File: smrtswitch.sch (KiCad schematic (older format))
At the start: 8 parts, among them J1 Screw_Terminal_01x02, J2 Conn_01x08, J3 Conn_01x03, J4 Conn_01x03, J5 Conn_01x03, J6 Conn_01x03

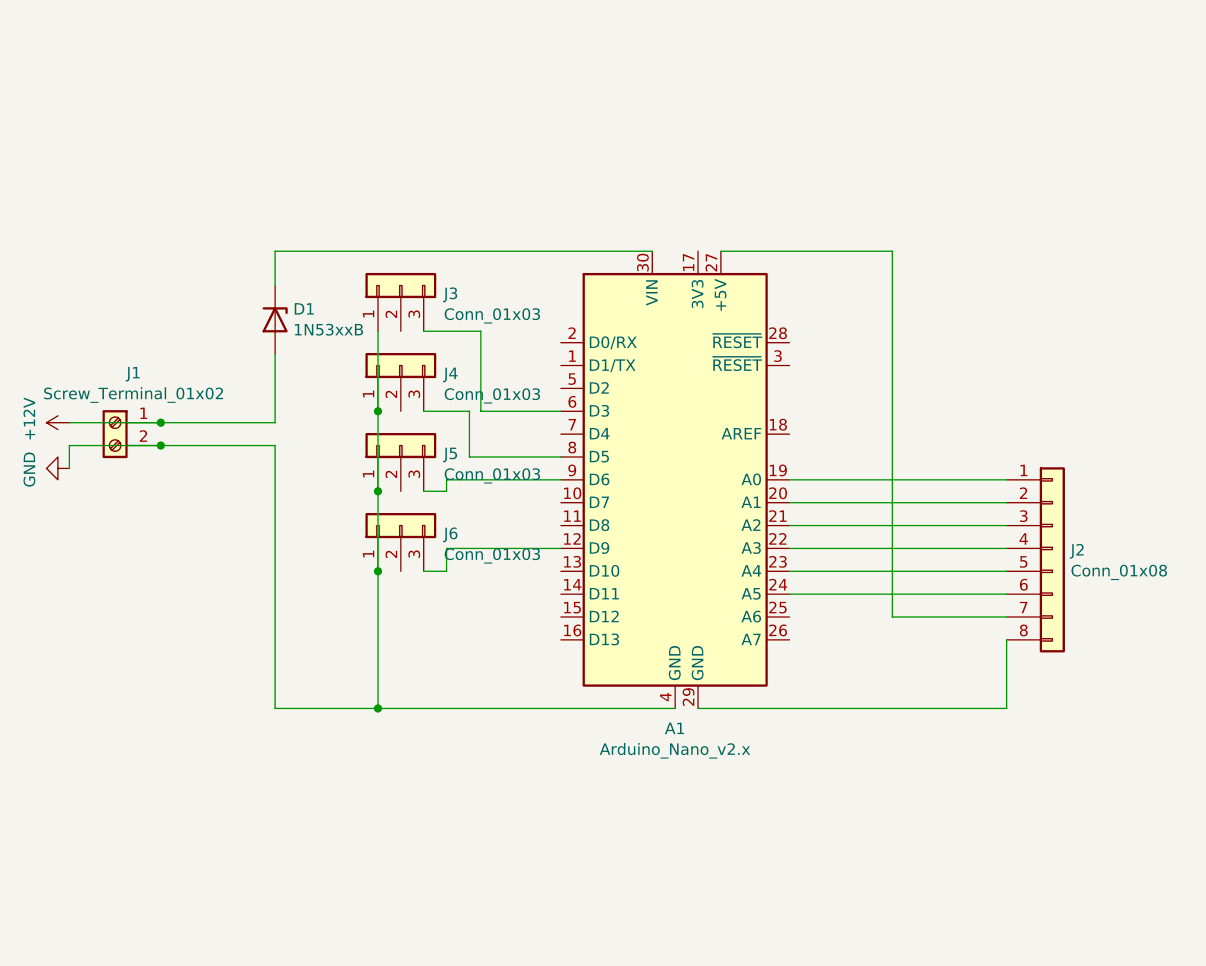
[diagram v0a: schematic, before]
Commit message: long-uncommitted changes
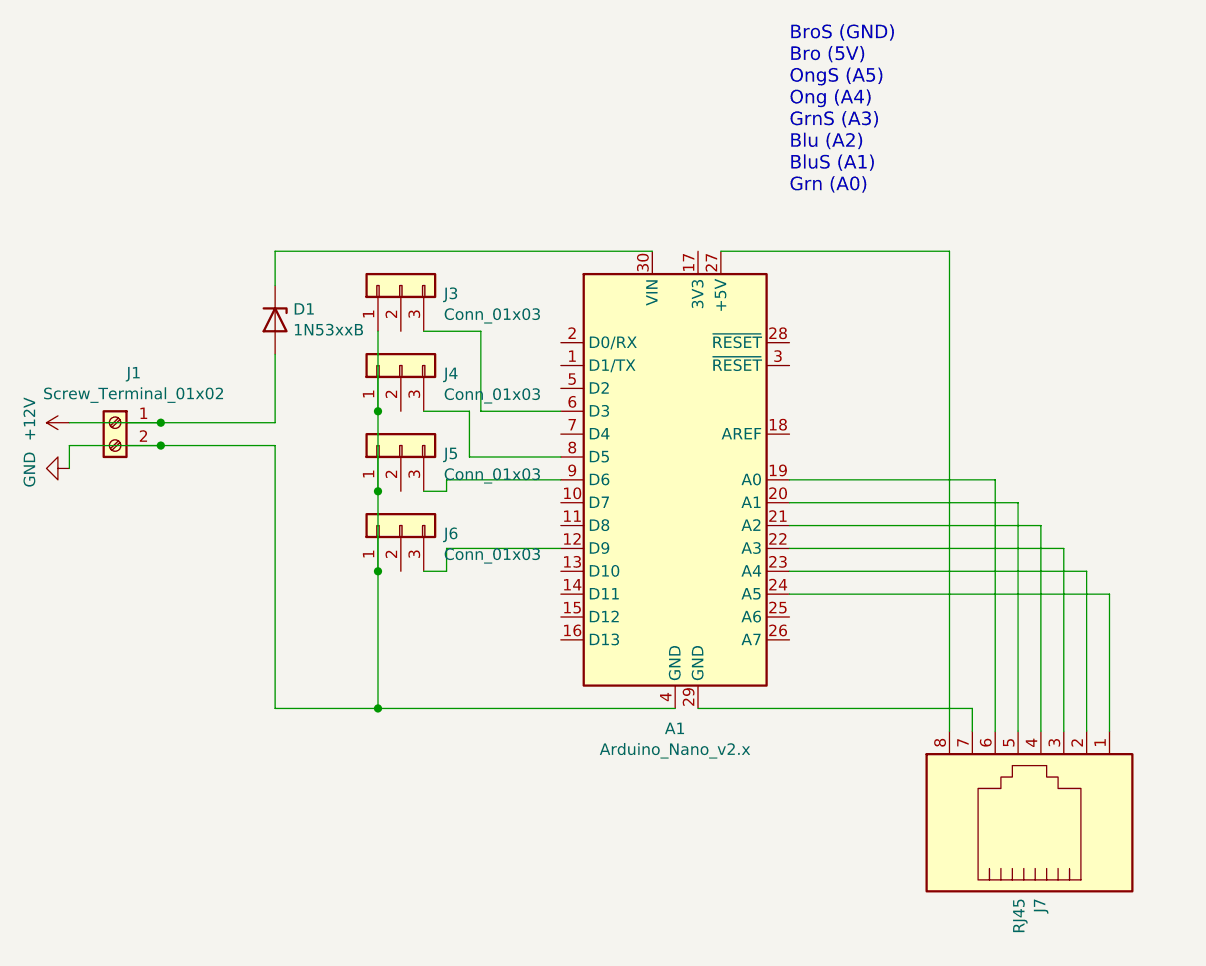
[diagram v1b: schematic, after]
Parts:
- removed J2: Conn_01x08, Connector_PinHeader_2.54mm:PinHeader_1x08_P2.54mm_Vertical, symbol Connector_Generic:Conn_01x08
- added J7: RJ45, Connector_RJ:RJ45_Amphenol_54602-x08_Horizontal, symbol Connector:RJ45
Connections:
- net at A1.19 (A0): now also J7.6
- net at A1.20 (A1): now also J7.5
- net at A1.21 (A2): now also J7.4
- net at A1.22 (A3): now also J7.3
- net at A1.23 (A4): now also J7.2
- net at A1.24 (A5): now also J7.1
- net at A1.27 (+5V): now also J7.8
- net at A1.29 (GND): now also J7.7
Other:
- note added: "BroS (GND)\nBro (5V)\nOngS (A5)\nOng (A4)\nGrnS (A3)\nBlu (A2)\nBluS (A1)\nGrn (A0)"
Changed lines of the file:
@@
 $EndComp
-$Comp
-L Connector_Generic:Conn_01x08 J2
-U 1 1 5E218367
-P 7100 3800
-F 0 "J2" H 7180 3792 50  0000 L CNN
-F 1 "Conn_01x08" H 7180 3701 50  0000 L CNN
-F 2 "Connector_PinHeader_2.54mm:PinHeader_1x08_P2.54mm_Vertical" H 7100 3800 50  0001 C CNN
-F 3 "~" H 7100 3800 50  0001 C CNN
-	1    7100 3800
-	1    0    0    -1
-$EndComp
-Wire Wire Line
-	5950 3500 6900 3500
-Wire Wire Line
-	6900 3600 5950 3600
-Wire Wire Line
-	5950 3700 6900 3700
-Wire Wire Line
-	6900 3800 5950 3800
-Wire Wire Line
-	5950 3900 6900 3900
-Wire Wire Line
-	6900 4000 5950 4000
-Wire Wire Line
-	5550 4500 6900 4500
-Wire Wire Line
-	6900 4500 6900 4200
-Wire Wire Line
-	5650 2500 6400 2500
-Wire Wire Line
-	6400 2500 6400 4100
-Wire Wire Line
-	6400 4100 6900 4100
 $Comp
 L Connector:Screw_Terminal_01x02 J1
@@
 Wire Wire Line
 	4150 3900 4150 4500
+$Comp
+L Connector:RJ45 J7
+U 1 1 5EEEE824
+P 7050 5000
+F 0 "J7" H 6720 5004 50  0000 R CNN
+F 1 "RJ45" H 6720 5095 50  0000 R CNN
+F 2 "Connector_RJ:RJ45_Amphenol_54602-x08_Horizontal" V 7050 5025 50  0001 C CNN
+F 3 "~" V 7050 5025 50  0001 C CNN
+	1    7050 5000
+	0    -1   -1   0
+$EndComp
+Text Notes 5950 2250 0    59   ~ 0
+BroS (GND)\nBro (5V)\nOngS (A5)\nOng (A4)\nGrnS (A3)\nBlu (A2)\nBluS (A1)\nGrn (A0)
+Wire Wire Line
+	6750 4600 6750 4500
+Wire Wire Line
+	6750 4500 5550 4500
+Wire Wire Line
+	5650 2500 6650 2500
+Wire Wire Line
+	6650 2500 6650 4600
+Wire Wire Line
+	7350 4600 7350 4000
+Wire Wire Line
+	7350 4000 5950 4000
+Wire Wire Line
+	7250 4600 7250 3900
+Wire Wire Line
+	7250 3900 5950 3900
+Wire Wire Line
+	7150 4600 7150 3800
+Wire Wire Line
+	7150 3800 5950 3800
+Wire Wire Line
+	7050 4600 7050 3700
+Wire Wire Line
+	7050 3700 5950 3700
+Wire Wire Line
+	6950 4600 6950 3600
+Wire Wire Line
+	6950 3600 5950 3600
+Wire Wire Line
+	6850 4600 6850 3500
+Wire Wire Line
+	6850 3500 5950 3500
 $EndSCHEMATC
